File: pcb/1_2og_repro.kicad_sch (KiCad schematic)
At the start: 219 parts, among them J1 Pico EzMate, J2 USB_B_Mini, J3 Raw Header, J4 JST PH S3B, Q1 2N7002, SW1 MX_SW_solder, SW10 MX_SW_solder, SW11 MX_SW_solder, SW12 MX_SW_solder, SW13 MX_SW_solder, SW14 MX_SW_solder, SW15 MX_SW_solder, SW16 MX_SW_solder, SW17 MX_SW_solder, SW18 MX_SW_solder, SW19 MX_SW_solder, SW2 MX_SW_solder, SW20 MX_SW_solder, SW21 MX_SW_solder, SW22 MX_SW_solder, SW23 MX_SW_solder, SW24 MX_SW_solder, SW25 MX_SW_solder, SW26 MX_SW_solder, SW27 MX_SW_solder, SW28 MX_SW_solder, SW29 MX_SW_solder, SW3 MX_SW_solder, SW30 MX_SW_solder, SW31 MX_SW_solder, SW32 MX_SW_solder, SW33 MX_SW_solder, SW34 MX_SW_solder, SW35 MX_SW_solder, SW36 MX_SW_solder, SW37 MX_SW_solder, SW38 MX_SW_solder, SW39 MX_SW_solder, SW4 MX_SW_solder, SW40 MX_SW_solder, SW41 MX_SW_solder, SW42 MX_SW_solder, SW43 MX_SW_solder, SW44 MX_SW_solder, SW45 MX_SW_solder, SW46 MX_SW_solder, SW47 MX_SW_solder, SW48 MX_SW_solder, SW49 MX_SW_solder, SW5 MX_SW_solder, SW50 MX_SW_solder, SW51 MX_SW_solder, SW52 MX_SW_solder, SW53 MX_SW_solder, SW54 MX_SW_solder, SW55 MX_SW_solder, SW56 MX_SW_solder, SW57 MX_SW_solder, SW58 MX_SW_solder, SW59 MX_SW_solder, SW6 MX_SW_solder, SW60 MX_SW_solder, SW61 MX_SW_solder, SW62 MX_SW_solder, SW63 MX_SW_solder, SW64 MX_SW_solder, SW65 MX_SW_solder, SW66 MX_SW_solder, SW67 MX_SW_solder, SW68 MX_SW_solder, SW69 MX_SW_solder, SW7 MX_SW_solder, SW70 MX_SW_solder, SW71 MX_SW_solder, SW72 MX_SW_solder, SW73 MX_SW_solder, SW74 MX_SW_solder, SW75 MX_SW_solder, SW76 MX_SW_solder, SW77 MX_SW_solder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

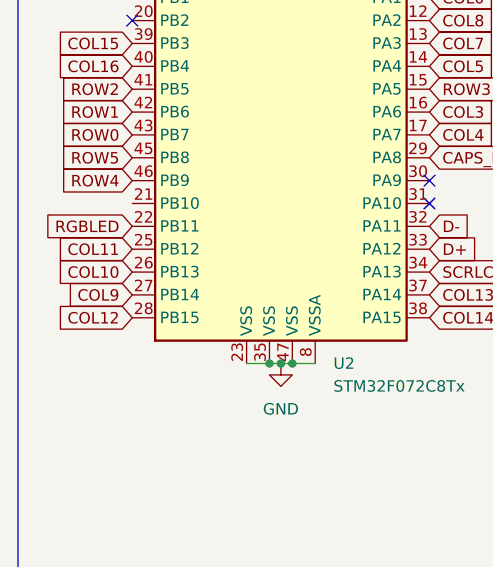
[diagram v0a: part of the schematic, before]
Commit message: routing improvements
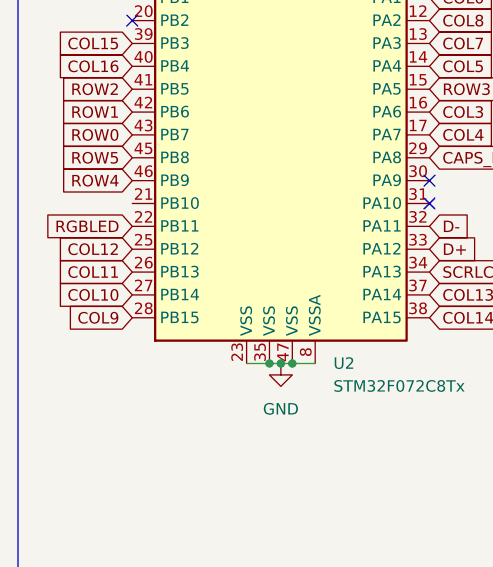
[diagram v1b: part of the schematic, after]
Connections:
- net COL10: now also U2.27 (PB14); no longer U2.26 (PB13)
- net COL11: now also U2.26 (PB13); no longer U2.25 (PB12)
- net COL12: now also U2.25 (PB12); no longer U2.28 (PB15)
- net COL9: now also U2.28 (PB15); no longer U2.27 (PB14)
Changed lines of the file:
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@@
     )
   )
-  (global_label "COL9" (shape input) (at 24.765 90.805 180) (fields_autoplaced)
+  (global_label "COL9" (shape input) (at 24.765 93.345 180) (fields_autoplaced)
     (effects (font (size 1.27 1.27)) (justify right))
-    (property "Intersheetrefs" "${INTERSHEET_REFS}" (at 17.0211 90.805 0)
+    (property "Intersheetrefs" "${INTERSHEET_REFS}" (at 17.0211 93.345 0)
       (effects (font (size 1.27 1.27)) (justify right) hide)
     )
@@
     )
   )
-  (global_label "COL10" (shape input) (at 24.765 88.265 180) (fields_autoplaced)
+  (global_label "COL10" (shape input) (at 24.765 90.805 180) (fields_autoplaced)
     (effects (font (size 1.27 1.27)) (justify right))
-    (property "Intersheetrefs" "${INTERSHEET_REFS}" (at 15.8116 88.265 0)
+    (property "Intersheetrefs" "${INTERSHEET_REFS}" (at 15.8116 90.805 0)
       (effects (font (size 1.27 1.27)) (justify right) hide)
     )
@@
     )
   )
-  (global_label "COL12" (shape input) (at 24.765 93.345 180) (fields_autoplaced)
-    (effects (font (size 1.27 1.27)) (justify right))
-    (property "Intersheetrefs" "${INTERSHEET_REFS}" (at 15.8116 93.345 0)
-      (effects (font (size 1.27 1.27)) (justify right) hide)
-    )
-  )
-  (global_label "COL11" (shape input) (at 24.765 85.725 180) (fields_autoplaced)
+  (global_label "COL12" (shape input) (at 24.765 85.725 180) (fields_autoplaced)
     (effects (font (size 1.27 1.27)) (justify right))
     (property "Intersheetrefs" "${INTERSHEET_REFS}" (at 15.8116 85.725 0)
       (effects (font (size 1.27 1.27)) (justify right) hide)
     )
+  )
+  (global_label "COL11" (shape input) (at 24.765 88.265 180) (fields_autoplaced)
+    (effects (font (size 1.27 1.27)) (justify right))
+    (property "Intersheetrefs" "${INTERSHEET_REFS}" (at 15.8116 88.265 0)
+      (effects (font (size 1.27 1.27)) (justify right) hide)
+    )
